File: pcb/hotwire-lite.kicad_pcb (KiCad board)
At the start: 2 copper layers, 60 x 32 mm, 26 parts, among them J1 Barrel_Jack, J2 Screw_Terminal_01x02, J3 Conn_01x04, J4 Conn_01x02, Q1 Si4162DY, SW1 SW_Push, U1 AP1117-50, U2 ATtiny402-SS, U3 INA181

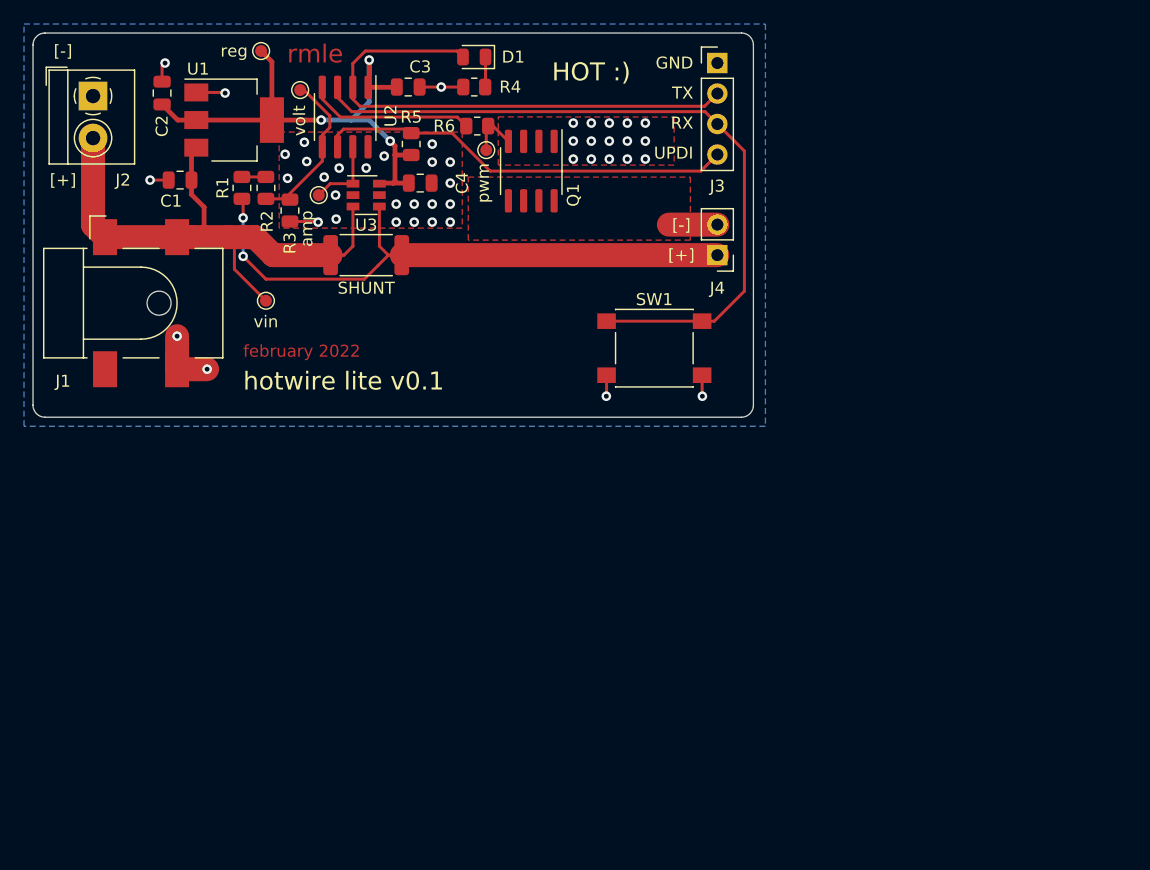
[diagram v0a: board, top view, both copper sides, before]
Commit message: added new v1.0 hardware design
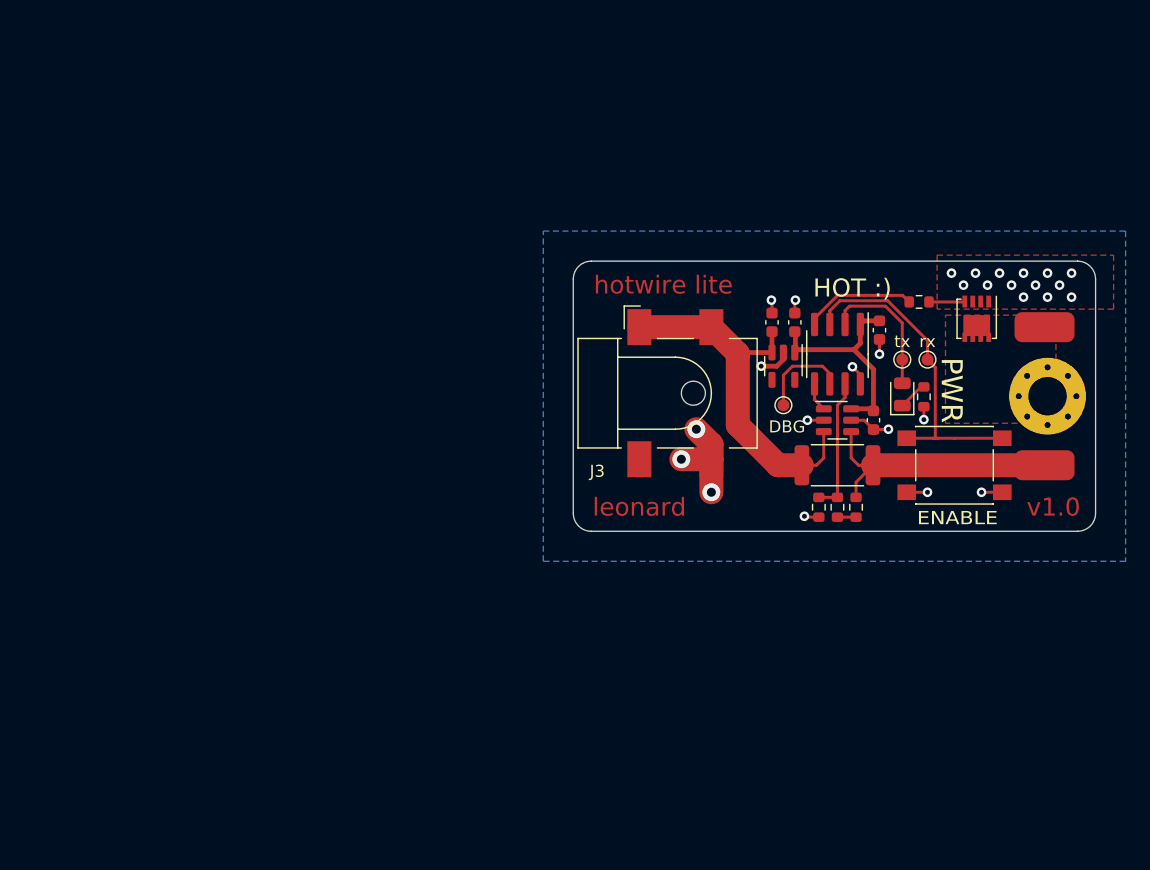
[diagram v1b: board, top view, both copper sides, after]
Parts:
- removed J4: Conn_01x02, Connector_PinHeader_2.54mm:PinHeader_1x02_P2.54mm_Vertical
- removed SHUNT: R_Small_US, Resistor_SMD:R_2512_6332Metric
- removed amp: amp, TestPoint:TestPoint_Pad_D1.0mm
- removed pwm: pwm, TestPoint:TestPoint_Pad_D1.0mm
- removed reg: reg, TestPoint:TestPoint_Pad_D1.0mm
- removed vin: vin, TestPoint:TestPoint_Pad_D1.0mm
- removed volt: volt, TestPoint:TestPoint_Pad_D1.0mm
- added H1: MountingHole_Pad, MountingHole:MountingHole_3.2mm_M3_Pad_Via, F.Cu at (149.5, 88.8)
- added TP6: DBG, TestPoint:TestPoint_Pad_D1.0mm, F.Cu at (127.5, 89.5)
- added TP7: rx, TestPoint:TestPoint_Pad_D1.0mm, F.Cu at (139.5, 85.7)
- added TP8: tx, TestPoint:TestPoint_Pad_D1.0mm, F.Cu at (137.4, 85.7)
- C1, C2, C4: footprint Capacitor_SMD:C_0805_2012Metric -> Capacitor_SMD:C_0603_1608Metric
- C3: value 0.1uF -> 0.01uF; footprint Capacitor_SMD:C_0805_2012Metric -> Capacitor_SMD:C_0603_1608Metric
- J1: value Barrel_Jack -> wire_pos; footprint Connector_BarrelJack:BarrelJack_CLIFF_FC681465S_SMT_Horizontal -> hotwire-lite:Wire Solder Pad
- J2: value Screw_Terminal_01x02 -> wire_neg; footprint TerminalBlock_4Ucon:TerminalBlock_4Ucon_1x02_P3.50mm_Horizontal -> hotwire-lite:Wire Solder Pad
- J3: value Conn_01x04 -> Barrel_Jack; footprint Connector_PinHeader_2.54mm:PinHeader_1x04_P2.54mm_Vertical -> Connector_BarrelJack:BarrelJack_CLIFF_FC681465S_SMT_Horizontal
- Q1: value Si4162DY -> SIRA18ADP; footprint Package_SO:SOIC-8_3.9x4.9mm_P1.27mm -> Package_SO:Vishay_PowerPAK_1212-8_Single
- R1, R2, R3, R5: value 10k -> 1k; footprint Resistor_SMD:R_0805_2012Metric -> Resistor_SMD:R_0603_1608Metric
- R4: value 220 -> 1k; footprint Resistor_SMD:R_0805_2012Metric -> Resistor_SMD:R_0603_1608Metric
- R6: value 220 -> 0.050; footprint Resistor_SMD:R_0805_2012Metric -> Resistor_SMD:R_2512_6332Metric
- U1: value AP1117-50 -> NCP716B; footprint Package_TO_SOT_SMD:SOT-223-3_TabPin2 -> Package_TO_SOT_SMD:SOT-23-5
- U3: value INA181 -> INA181A1
- moved J2 81.6 mm to (149.2, 83.0), turned to 0 degrees
- moved J1 76.5 mm to (149.2, 94.5)
- moved R1 57.7 mm to (133.6, 98.0), turned to -90 degrees
- moved C2 56.1 mm to (128.4, 82.6)
- moved R2 54.5 mm to (132.0, 98.0), turned to 90 degrees
- moved C1 50.7 mm to (126.5, 82.6), turned to 90 degrees
- moved R3 50.5 mm to (130.4, 98.0)
- moved U1 50.1 mm to (127.5, 86.2), turned to -90 degrees
- moved C3 47.7 mm to (135.0, 90.8), turned to -90 degrees
- moved U2 45.5 mm to (132.0, 85.2)
- moved R4 45.5 mm to (139.2, 88.8), turned to -90 degrees
- moved D1 45.4 mm to (137.4, 88.6), turned to 90 degrees
- moved R5 44.3 mm to (138.8, 80.9), turned to 0 degrees
- moved U3 43.5 mm to (132.0, 90.8)
- moved R6 41.2 mm to (132.0, 94.5)
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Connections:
- C1 pad 2: GNDREF -> GND
- C2 pad 1: /vcc -> +5V
- C2 pad 2: GNDREF -> GND
- C3 pad 1: /vcc -> +5V
- C3 pad 2: GNDREF -> GND
- C4 pad 1: /vcc -> +5V
- C4 pad 2: GNDREF -> GND
- J1 pad 1: /vin -> /shunt_low
- J2 pad 1: GNDREF -> /load_neg
- J3 pad 1: GNDREF -> /vin
- J3 pad 2: /tx_led -> GND
- J3 pad 3: /rx_button -> (no net)
- Q1 pad 1: GNDREF -> GND
- Q1 pad 2: GNDREF -> GND
- Q1 pad 3: GNDREF -> GND
- Q1 pad 5: /output_return -> /load_neg
- R3 pad 2: GNDREF -> GND
- R4 pad 2: GNDREF -> GND
- R5 pad 1: /vcc -> /pwm_output
- R5 pad 2: /UPDI -> Net-(Q1-Pad4)
- R6 pad 1: /pwm_output -> /vin
- R6 pad 2: Net-(Q1-Pad4) -> /shunt_low
- SW1 pad 2: GNDREF -> GND
- U1 pad 1: GNDREF -> +5V
- U1 pad 2: /vcc -> GND
- U2 pad 1: /vcc -> +5V
- U2 pad 5: /voltage_sense -> /current_sense
- U2 pad 7: /current_sense -> /voltage_sense
- U2 pad 8: GNDREF -> GND
- U3 pad 2: GNDREF -> GND
- U3 pad 5: GNDREF -> GND
- U3 pad 6: /vcc -> +5V
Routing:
- net /vcc: track 44.7 -> 0.00 mm, vias 3 -> 0
- net /rx_button: track 60.8 -> 27.4 mm
- net /tx_led: track 43.8 -> 11.7 mm
- net /shunt_low: track 50.3 -> 21.8 mm, vias 2 -> 0
- net /UPDI: track 34.8 -> 7.79 mm
- net GND: track 0.00 -> 26.6 mm, vias 0 -> 28
- net GNDREF: track 21.4 -> 0.00 mm, vias 46 -> 0
- net /vin: track 49.5 -> 30.7 mm
- net +5V: track 0.00 -> 18.6 mm
- net /pwm_output: track 13.9 -> 9.41 mm
- net /output_return: track 4.04 -> 0.00 mm
- net /current_sense: track 6.32 -> 2.39 mm
- net /voltage_sense: track 13.7 -> 11.3 mm
- net Net-(Q1-Pad4): track 4.28 -> 3.00 mm
- added copper zone on F.Cu, net /load_neg
- added copper zone on B.Cu, net GND
- added copper zone on F.Cu, net GND
- removed copper zone on F.Cu, net /output_return
- removed copper zone on B.Cu, net GNDREF
- removed copper zone on F.Cu, net GNDREF
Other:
- board size 60 x 32 mm -> 43.5 x 22.5 mm
- net class Default removed
- net class VCC removed
- board text added: "#6 screw"
- board text added: "ENABLE"
- board text added: "PWR"
- board text added: "center +"
- board text added: "hotwire lite"
- board text added: "leonard"
- board text added: "v1.0"
- board text added: "vin: 12-24v vout: 1-100% vin"
- board text removed: "GND"
- board text removed: "RX"
- board text removed: "TX"
- board text removed: "UPDI"
- board text removed: "[+]"
- board text removed: "[-]"
- board text removed: "february 2022"
- board text removed: "hotwire lite v0.1"
- board text removed: "rmle"

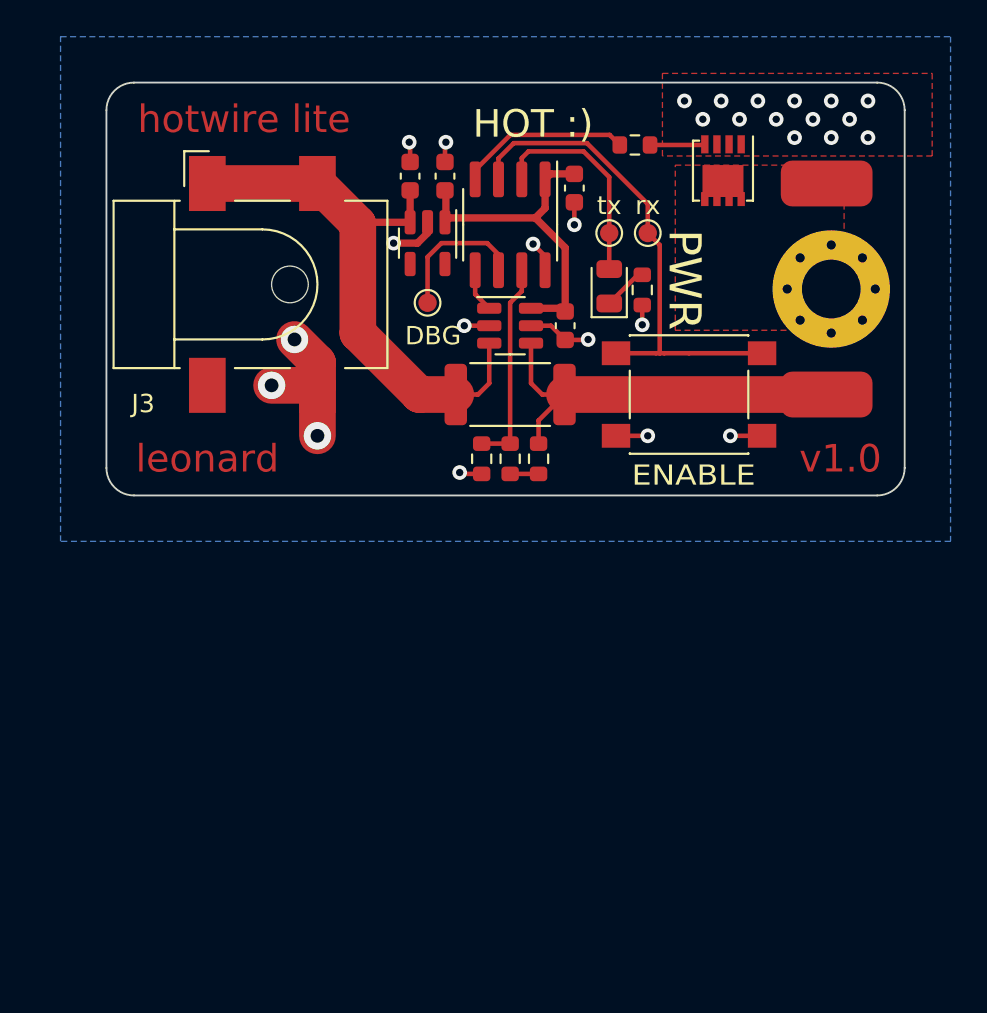
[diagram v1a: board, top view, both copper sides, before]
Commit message: v1.0 hardware
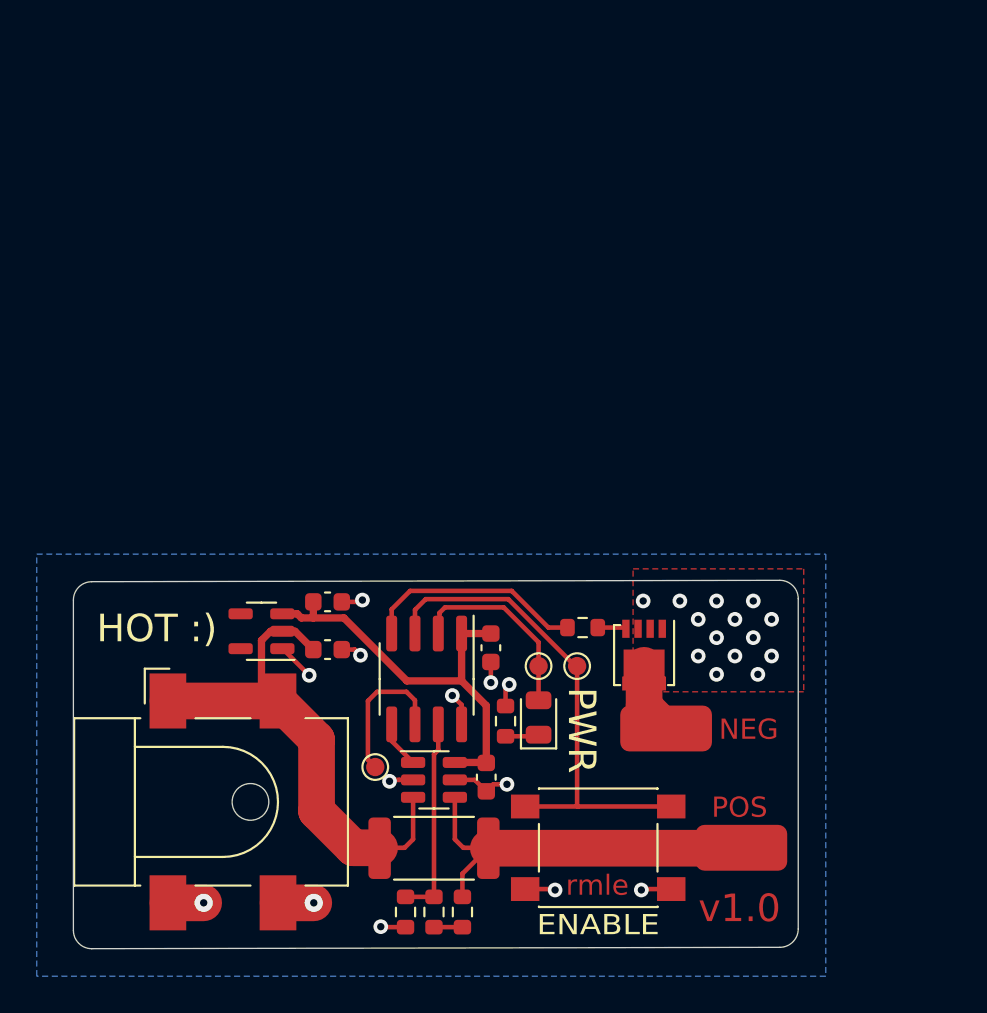
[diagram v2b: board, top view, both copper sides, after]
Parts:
- removed H1: MountingHole_Pad, MountingHole:MountingHole_3.2mm_M3_Pad_Via
- removed TP6: DBG, TestPoint:TestPoint_Pad_D1.0mm
- removed TP7: rx, TestPoint:TestPoint_Pad_D1.0mm
- removed TP8: tx, TestPoint:TestPoint_Pad_D1.0mm
- added TP1: TestPoint, TestPoint:TestPoint_Pad_D1.0mm, F.Cu at (124.7, 114.8)
- added TP2: TestPoint, TestPoint:TestPoint_Pad_D1.0mm, F.Cu at (135.7, 109.3)
- added TP3: TestPoint, TestPoint:TestPoint_Pad_D1.0mm, F.Cu at (133.6, 109.3)
- C3: value 0.01uF -> 0.1uF
- J1: value wire_pos -> Barrel_Jack_Switch_Pin3Ring; footprint hotwire-lite:Wire Solder Pad -> Connector_BarrelJack:BarrelJack_CLIFF_FC681465S_SMT_Horizontal
- J2: value wire_neg -> WIRE+; footprint hotwire-lite:Wire Solder Pad -> hotwire-lite:wire_solder_pad
- J3: value Barrel_Jack -> WIRE-; footprint Connector_BarrelJack:BarrelJack_CLIFF_FC681465S_SMT_Horizontal -> hotwire-lite:wire_solder_pad
- Q1: value SIRA18ADP -> SiRA18ADP
- U1: value NCP716B -> NCP716
- U3: value INA181A1 -> INA180A1
- moved J1 39.7 mm to (116.3, 116.7)
- moved J2 36.5 mm to (144.6, 119.2), turned to 90 degrees
- moved J3 32.7 mm to (140.5, 112.7), turned to 90 degrees
- moved C4 32.5 mm to (130.7, 115.3), turned to 90 degrees
- moved Q1 26.7 mm to (139.3, 108.7)
- moved R5 26.5 mm to (135.9, 107.2)
- moved C1 26.2 mm to (122.0, 108.4), turned to 0 degrees
- moved SW1 25.2 mm to (136.8, 119.2)
- moved U2 25.2 mm to (127.5, 110.0)
- moved U3 25.1 mm to (127.8, 115.5)
- moved R6 25.1 mm to (127.8, 119.2)
- moved R1 25.0 mm to (129.4, 122.7)
- moved R2 25.0 mm to (127.8, 122.7)
- moved R3 25.0 mm to (126.3, 122.7)
- moved R4 24.7 mm to (131.8, 112.3), turned to 90 degrees
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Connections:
- C3 pad 1: +5V -> GND
- C3 pad 2: GND -> +5V
- C4 pad 1: +5V -> GND
- C4 pad 2: GND -> +5V
- J1 pad 1: /shunt_low -> /vin
- J2 pad 1: /load_neg -> /wire_pos
- J3 pad 1: /vin -> /wire_neg
- Q1 pad 5: /load_neg -> /wire_neg
- R1 pad 1: /shunt_low -> /wire_pos
- R6 pad 2: /shunt_low -> /wire_pos
- U1 pad 1: +5V -> GND
- U1 pad 2: GND -> /vin
- U1 pad 3: /vin -> +5V
- U3 pad 4: /shunt_low -> /wire_pos
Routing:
- net /shunt_low: track 21.8 -> 0.00 mm
- net /wire_pos: track 0.00 -> 21.4 mm
- net GND: track 26.6 -> 21.7 mm, vias 28 -> 27
- net +5V: track 18.6 -> 23.0 mm
- net /wire_neg: track 0.00 -> 3.94 mm
- net /pwm_output: track 9.41 -> 12.1 mm
- net /vin: track 30.7 -> 28.6 mm
- net Net-(Q1-Pad4): track 3.00 -> 1.56 mm
- net /tx_led: track 11.7 -> 10.6 mm
- net Net-(D1-Pad1): track 2.45 -> 1.84 mm
- removed copper zone on F.Cu, net /load_neg
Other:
- board size 43.5 x 22.5 mm -> 39.5 x 20.1 mm
- board text added: "NEG"
- board text added: "POS"
- board text added: "april 2022 rmle"
- board text added: "hotwire lite vin: 12-24v vout: 1-100% vin"
- board text added: "rmle"
- board text removed: "#6 screw"
- board text removed: "center +"
- board text removed: "hotwire lite"
- board text removed: "leonard"
- board text removed: "vin: 12-24v vout: 1-100% vin"
